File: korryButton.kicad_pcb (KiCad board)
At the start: 2 copper layers, 30 x 30 mm, 15 parts, among them CN1 B2B-XH-A (LF)(SN), CN2 B2B-XH-A (LF)(SN), U1 SN74AHCT125DR, U2 B3B-XH-A(LF)(SN), U3 WS2811C, U4 WS2811C

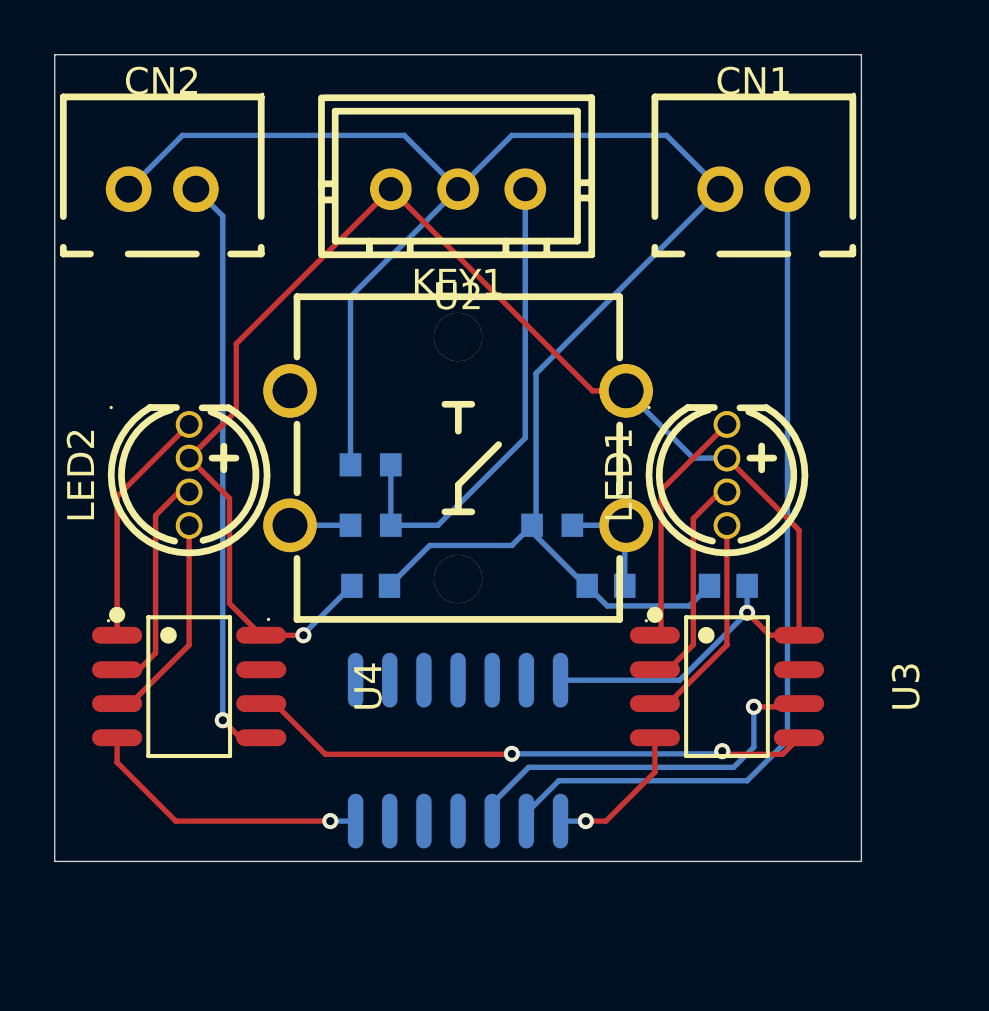
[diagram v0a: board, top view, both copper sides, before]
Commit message: update
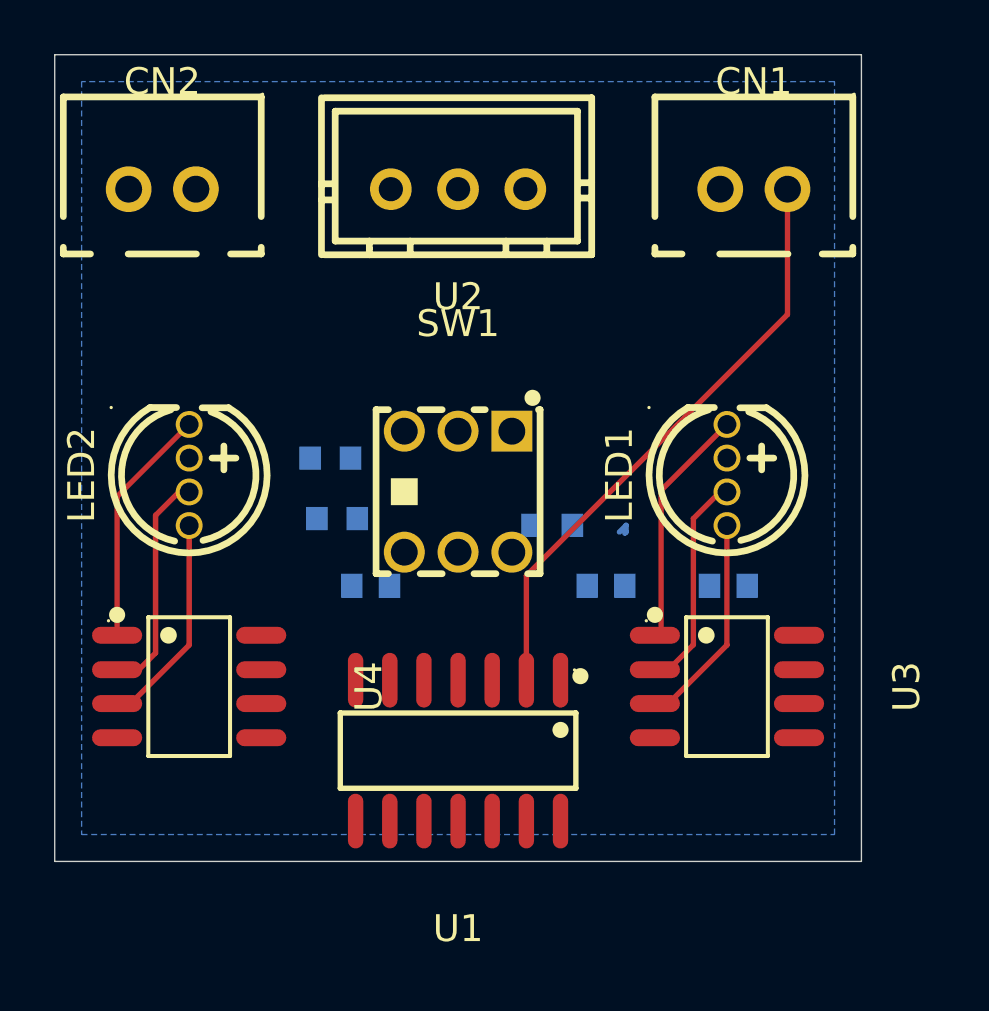
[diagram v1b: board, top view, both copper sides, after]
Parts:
- removed KEY1: ，12×12x7.3，:2.55N，:0.3mm, lcsc_footprints:C84931_KEY-TH_4P-L12_0-W12_0-P5_00-LS13_4-EH
- added SW1: 5.8 ZSGT, lcsc_footprints:C2681587_SW-TH_5_8ZSGT, F.Cu at (100.0, 126.2)
- U1: moved to F.Cu
- moved R3 1.52 mm to (95.2, 125.0)
- moved R2 1.27 mm to (95.5, 127.2)
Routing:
- net GND: track 83.1 -> 0.00 mm, vias 2 -> 0
- net VCC: track 60.6 -> 0.00 mm, vias 2 -> 0
- net Net-(U4-DO): track 21.9 -> 0.00 mm, vias 1 -> 0
- net Net-(U3-DO): track 21.1 -> 0.00 mm, vias 2 -> 0
- net Net-(R2-Pad1): track 17.8 -> 0.00 mm
- net Net-(U1-1Y): track 14.5 -> 0.00 mm, vias 1 -> 0
- net Net-(U1-1A): track 31.6 -> 22.3 mm
- net Net-(C1-Pad1): track 4.62 -> 0.67 mm
- net Net-(R2-Pad2): track 2.25 -> 0.00 mm
- added copper zone on B.Cu, net GND
